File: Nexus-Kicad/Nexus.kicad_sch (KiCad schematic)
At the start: 15 parts, among them J1 Conn_01x02_Socket

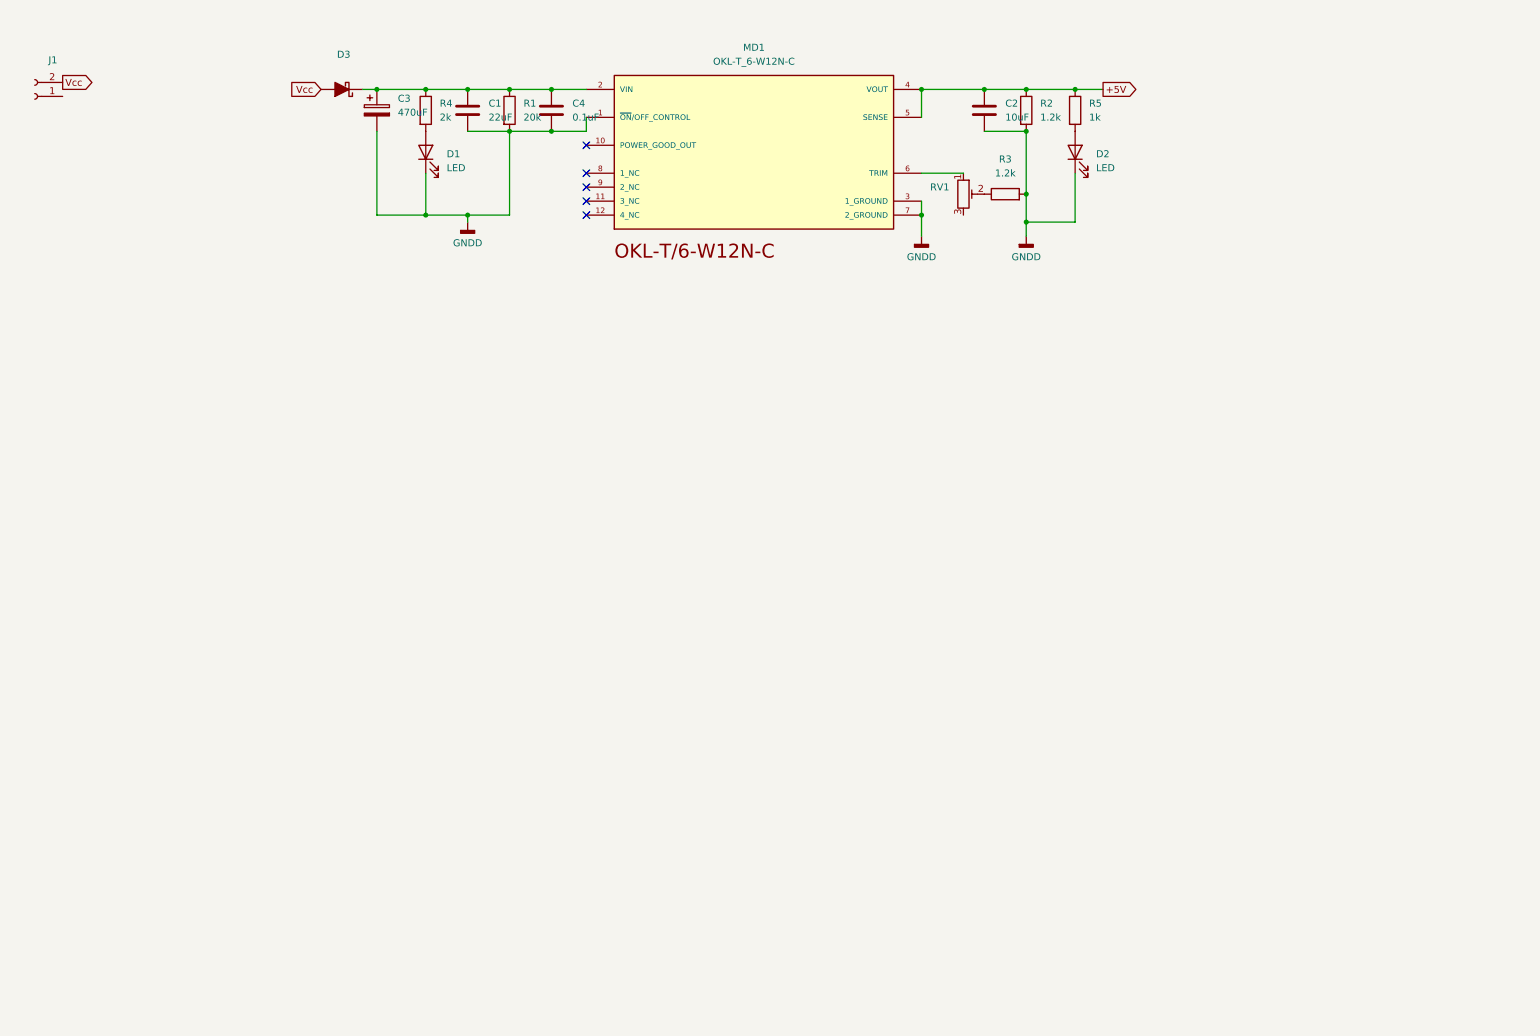
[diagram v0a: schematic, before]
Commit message: EDA ver 1.0
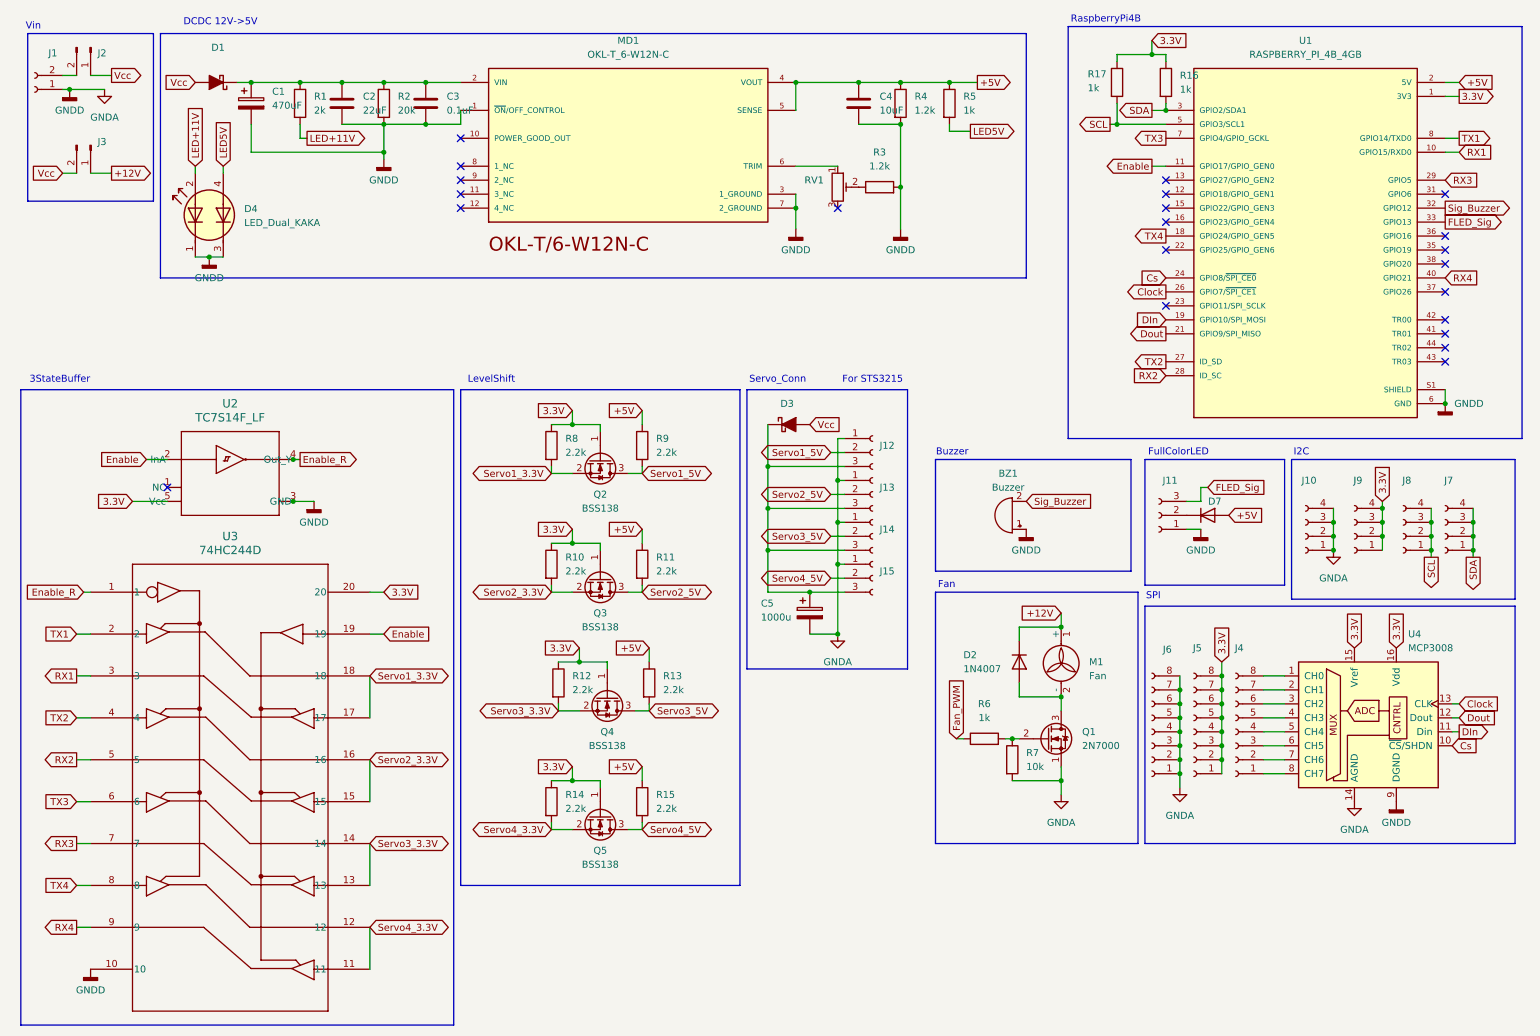
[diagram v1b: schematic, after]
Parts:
- removed D1, D2: LED, LED_SMD:LED_0603_1608Metric_Pad1.05x0.95mm_HandSolder, symbol Device:LED
- added BZ1: Buzzer, symbol Device:Buzzer
- added C5: 1000u, symbol Device:C_Polarized
- added D2: 1N4007, Diode_THT:D_DO-41_SOD81_P10.16mm_Horizontal, symbol Diode:1N4007
- added D3: D_Schottky_Filled, Diode_THT:D_DO-201AD_P12.70mm_Horizontal, symbol Device:D_Schottky_Filled
- added D4: LED_Dual_KAKA, LED_SMD:LED_Kingbright_KPBD-3224, symbol Device:LED_Dual_KAKA
- added D7: D, Diode_THT:D_DO-34_SOD68_P7.62mm_Horizontal, symbol Device:D
- added J10, J7, J8, J9: Conn_01x04_Socket, symbol Connector:Conn_01x04_Socket
- added J11: Conn_01x03_Socket, Connector_PinSocket_2.54mm:PinSocket_1x03_P2.54mm_Vertical, symbol Connector:Conn_01x03_Socket
- added J12, J13, J14, J15: Conn_01x03_Socket, Connector_Molex:Molex_SPOX_5267-03A_1x03_P2.50mm_Vertical, symbol Connector:Conn_01x03_Socket
- added J2, J3: Conn_01x02_Pin, Connector_AMASS:AMASS_XT30U-F_1x02_P5.0mm_Vertical, symbol Connector:Conn_01x02_Pin
- added J4, J5, J6: Conn_01x08_Socket, symbol Connector:Conn_01x08_Socket
- added M1: Fan, symbol Motor:Fan
- added Q1: 2N7000, Package_TO_SOT_THT:TO-92_Inline, symbol Transistor_FET:2N7000
- added Q2, Q3, Q4, Q5: BSS138, Package_TO_SOT_SMD:SOT-23, symbol Transistor_FET:BSS138
- added R10, R11, R12, R13, R14, R15, R8, R9: 2.2k, Resistor_SMD:R_0603_1608Metric, symbol Device:R
- added R16, R17, R6: 1k, Resistor_SMD:R_0603_1608Metric, symbol Device:R
- added R7: 10k, Resistor_SMD:R_0603_1608Metric, symbol Device:R
- added U1: RASPBERRY_PI_4B_4GB, RaspberryPi4B:MODULE_RASPBERRY_PI_4B_4GB, symbol RASPBERRY_PI_4B_4GB:RASPBERRY_PI_4B_4GB
- added U2: TC7S14F_LF, SOT-25 SMV_TOS, symbol Tc7S14F:TC7S14F_LF
- added U3: 74HC244D, SOIC20_TOS, symbol 74HC244:74HC244D
- added U4: MCP3008, symbol Analog_ADC:MCP3008
- D1: renamed from D3; footprint (none) -> Diode_THT:D_DO-201AD_P12.70mm_Horizontal
- J1: footprint Connector_AMASS:AMASS_XT60-F_1x02_P7.20mm_Vertical -> Connector_AMASS:AMASS_XT30U-F_1x02_P5.0mm_Vertical
- MD1: footprint OKL-T_6-W12N-C:MURATA_OKL-T-6-W12N-C_0 -> OKLT6W12N:MURATA_OKL-T-6-W12N-C_0
- renumbered C3 to C1, C1 to C2, C4 to C3, C2 to C4, R4 to R1, R1 to R2, R2 to R4
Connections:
- net GNDD is gone; now on net GND: C1.2, C2.2, C3.2, C4.2, MD1.1 (~{ON}/OFF_CONTROL), MD1.3 (1_GROUND), MD1.7 (2_GROUND), R2.2, R3.2, R4.2
- net Vcc: now also D3.2 (A), J2.1 (Pin_1), J3.2 (Pin_2); no longer J1.2 (Pin_2)
- net LED+11V: now reaches R1.2
- net LED+11V: now also D4.2 (A1)
- net GND: now reaches J1.1 (Pin_1)
- net GND: now also BZ1.1 (+), C5.2, D4.1 (K1), D4.3 (K2), J10.1 (Pin_1), J10.2 (Pin_2), J10.3 (Pin_3), J10.4 (Pin_4), J11.1 (Pin_1), J12.1 (Pin_1), J13.1 (Pin_1), J14.1 (Pin_1), J15.1 (Pin_1), J6.1 (Pin_1), J6.2 (Pin_2), J6.3 (Pin_3), J6.4 (Pin_4), J6.5 (Pin_5), J6.6 (Pin_6), J6.7 (Pin_7), J6.8 (Pin_8), Q1.1 (S), R7.2, U1.14 (GND), U1.20 (GND), U1.25 (GND), U1.30 (GND), U1.34 (GND), U1.39 (GND), U1.6 (GND), U1.9 (GND), U1.S1 (SHIELD), U1.S2 (SHIELD), U1.S3 (SHIELD), U1.S4 (SHIELD), U2.3 (GND), U3.10, U4.14 (AGND), U4.9 (DGND)
- net LED5V: now reaches R5.2
- net LED5V: now also D4.4 (A2)
- net +5V renamed 5V
- net 5V: now also D7.2 (A), R11.1, R13.1, R15.1, R9.1, U1.2 (5V), U1.4 (5V)
- new net: D7.1 (K), J11.2 (Pin_2)
- new net: J4.1 (Pin_1), U4.8 (CH7)
- new net: J4.2 (Pin_2), U4.7 (CH6)
- new net: J4.3 (Pin_3), U4.6 (CH5)
- new net: J4.4 (Pin_4), U4.5 (CH4)
- new net: J4.5 (Pin_5), U4.4 (CH3)
- new net: J4.6 (Pin_6), U4.3 (CH2)
- new net: J4.7 (Pin_7), U4.2 (CH1)
- new net: J4.8 (Pin_8), U4.1 (CH0)
- new net: D2.2 (A), M1.2 (-), Q1.3 (D)
- new net: J1.2 (Pin_2), J2.2 (Pin_2)
- new net: Q1.2 (G), R6.2, R7.1
- new net: C5.1, D3.1 (K), J12.3 (Pin_3), J13.3 (Pin_3), J14.3 (Pin_3), J15.3 (Pin_3)
- new net +12V: D2.1 (K), J3.1 (Pin_1), M1.1 (+)
- new net 3V3: J5.1 (Pin_1), J5.2 (Pin_2), J5.3 (Pin_3), J5.4 (Pin_4), J5.5 (Pin_5), J5.6 (Pin_6), J5.7 (Pin_7), J5.8 (Pin_8), J9.1 (Pin_1), J9.2 (Pin_2), J9.3 (Pin_3), J9.4 (Pin_4), Q2.1 (G), Q3.1 (G), Q4.1 (G), Q5.1 (G), R10.1, R12.1, R14.1, R16.1, R17.1, R8.1, U1.1 (3V3), U1.17 (3V3), U3.20, U4.15 (Vref), U4.16 (Vdd)
- new net Clock: U1.26 (GPIO7/~{SPI_CE1}), U4.13 (CLK)
- new net Cs: U1.24 (GPIO8/~{SPI_CE0}), U4.10 (~{CS}/SHDN)
- new net DIn: U1.19 (GPIO10/SPI_MOSI), U4.11 (Din)
- new net Dout: U1.21 (GPIO9/SPI_MISO), U4.12 (Dout)
- new net Enable: U1.11 (GPIO17/GPIO_GEN0), U2.2 (InA), U3.19
- new net Enable_R: U2.4 (Out_Y), U3.1
- new net FLED_Sig: J11.3 (Pin_3), U1.33 (GPIO13)
- new net Fan_PWM: R6.1
- new net RX1: U1.10 (GPIO15/RXD0), U3.3
- new net RX2: U1.28 (ID_SC), U3.5
- new net RX3: U1.29 (GPIO5), U3.7
- new net RX4: U1.40 (GPIO21), U3.9
- new net SCL: J8.1 (Pin_1), J8.2 (Pin_2), J8.3 (Pin_3), J8.4 (Pin_4), R17.2, U1.5 (GPIO3/SCL1)
- new net SDA: J7.1 (Pin_1), J7.2 (Pin_2), J7.3 (Pin_3), J7.4 (Pin_4), R16.2, U1.3 (GPIO2/SDA1)
- new net Servo1_3.3V: Q2.2 (S), R8.2, U3.17, U3.18
- new net Servo1_5V: J12.2 (Pin_2), Q2.3 (D), R9.2
- new net Servo2_3.3V: Q3.2 (S), R10.2, U3.15, U3.16
- new net Servo2_5V: J13.2 (Pin_2), Q3.3 (D), R11.2
- new net Servo3_3.3V: Q4.2 (S), R12.2, U3.13, U3.14
- new net Servo3_5V: J14.2 (Pin_2), Q4.3 (D), R13.2
- new net Servo4_3.3V: Q5.2 (S), R14.2, U3.11, U3.12
- new net Servo4_5V: J15.2 (Pin_2), Q5.3 (D), R15.2
- new net Sig_Buzzer: BZ1.2 (-), U1.32 (GPIO12)
- new net TX1: U1.8 (GPIO14/TXD0), U3.2
- new net TX2: U1.27 (ID_SD), U3.4
- new net TX3: U1.7 (GPIO4/GPIO_GCKL), U3.6
- new net TX4: U1.18 (GPIO24/GPIO_GEN5), U3.8
- no-connect marks 5 -> 22
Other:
- note added: "3StateBuffer"
- note added: "Buzzer"
- note added: "DCDC 12V->5V"
- note added: "Fan"
- note added: "For STS3215"
- note added: "FullColorLED"
- note added: "I2C"
- note added: "LevelShift"
- note added: "RaspberryPi4B"
- note added: "SPI"
- note added: "Servo_Conn"
- note added: "Vin"
- company: (none) -> RMF-HRU-Kamada Takuya
- title: (none) -> B.T.F-Nexus
- moved on the sheet: C1, C2, C3, C4, D1, J1, MD1, R1, R2, R3, R4, R5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
